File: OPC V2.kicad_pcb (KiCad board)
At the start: 4 copper layers, 65 x 43 mm, 57 parts, among them J1 691382010004, J2 691382010004, J3 MEC1-110-02-F-D-A, J4 691382010004, J5 Conn_01x05, J6 Conn_01x04_Pin, U1 TS3A4751PWR, U2 TS3A4751PWR, U3 MCP23017x-x-ML, U4 TS3A4751PWR, U5 ADS1120-PW, U6 TS3A4751PWR, U7 BMP581, U8 DS3231MZ, U9 TS3A4751PWR

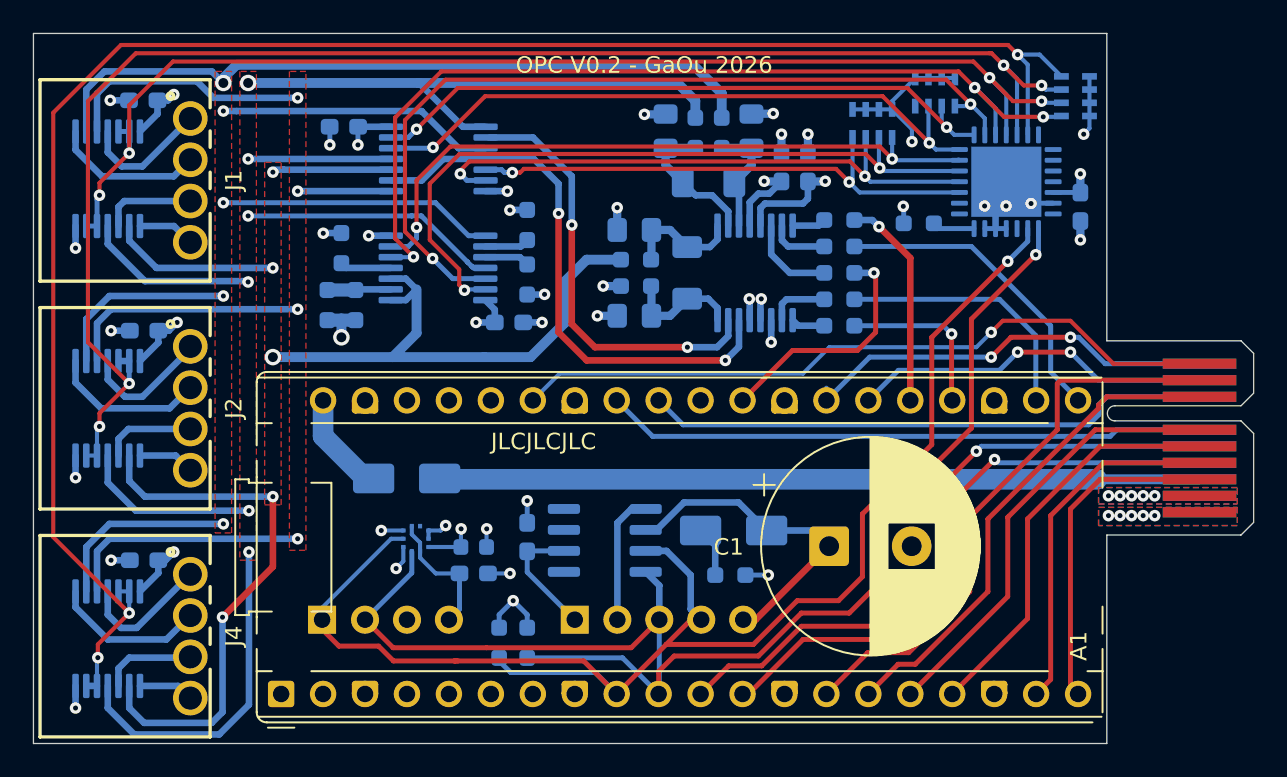
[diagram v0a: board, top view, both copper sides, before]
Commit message: avant prod
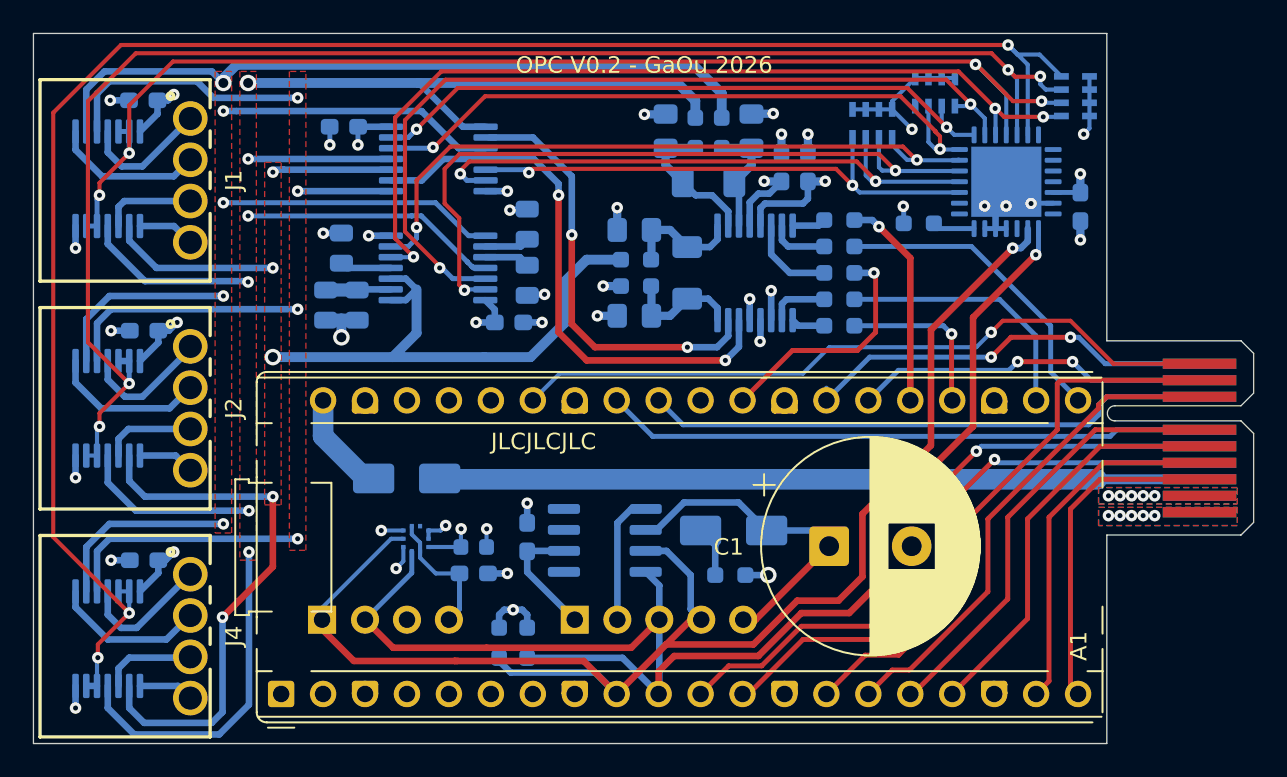
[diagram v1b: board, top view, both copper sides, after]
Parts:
- C10, C11, C12, C2, C3, C4, C5, C6, C7, C8, C9: value 0.1µ -> 0.1µ 10V
- R10, R3, R5, R7, R9: footprint Resistor_SMD:R_0603_1608Metric_Pad0.98x0.95mm_HandSolder -> Resistor_SMD:R_0805_2012Metric
- moved R10 0.10 mm to (117.7, 116.5)
- moved R9 0.10 mm to (119.6, 116.5)
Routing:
- net /Entrées/RREF_16k5: track 56.3 -> 54.6 mm
- net /Entrées/2_WIRE: track 39.3 -> 40.6 mm
- net /Entrées/INPUT_1_EN: track 73.2 -> 74.4 mm
- net /Entrées/TC_VCC: track 40.7 -> 41.7 mm
- net /Entrées/INPUT_3_EN: track 108.7 -> 109.5 mm
- net /Entrées/4_WIRE: track 35.2 -> 35.9 mm
- net GND: track 68.6 -> 68.0 mm
